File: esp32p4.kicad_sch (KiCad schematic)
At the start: 19 parts, among them U3 TLV62569DBV

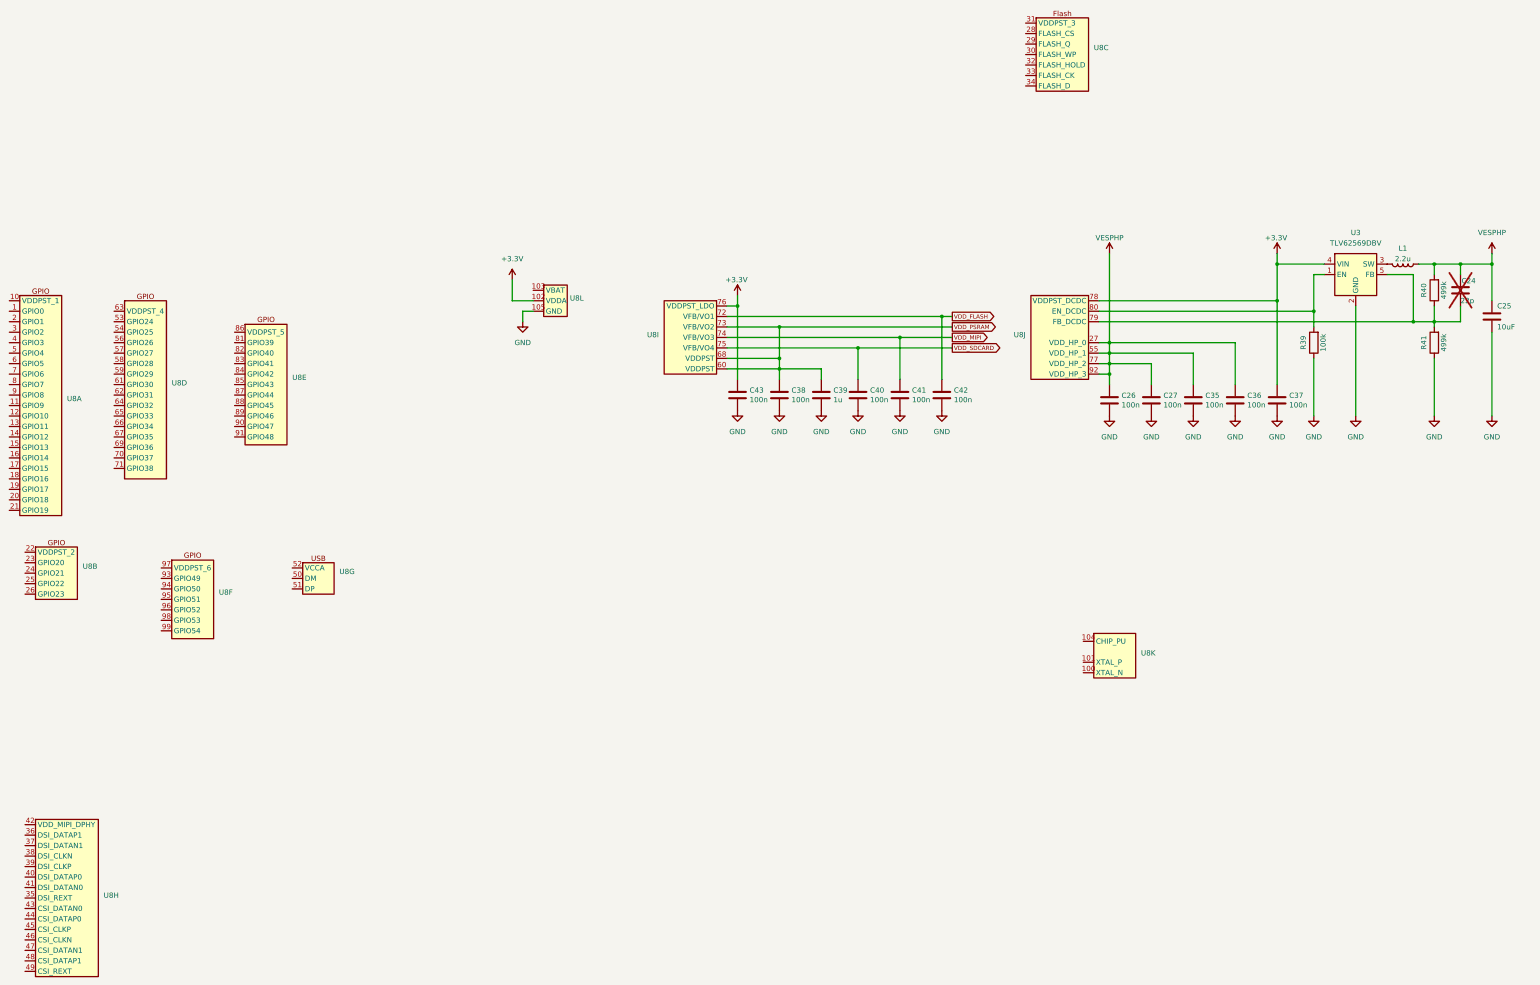
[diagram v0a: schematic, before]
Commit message: Mostly power related stuff for the ESP32-P4
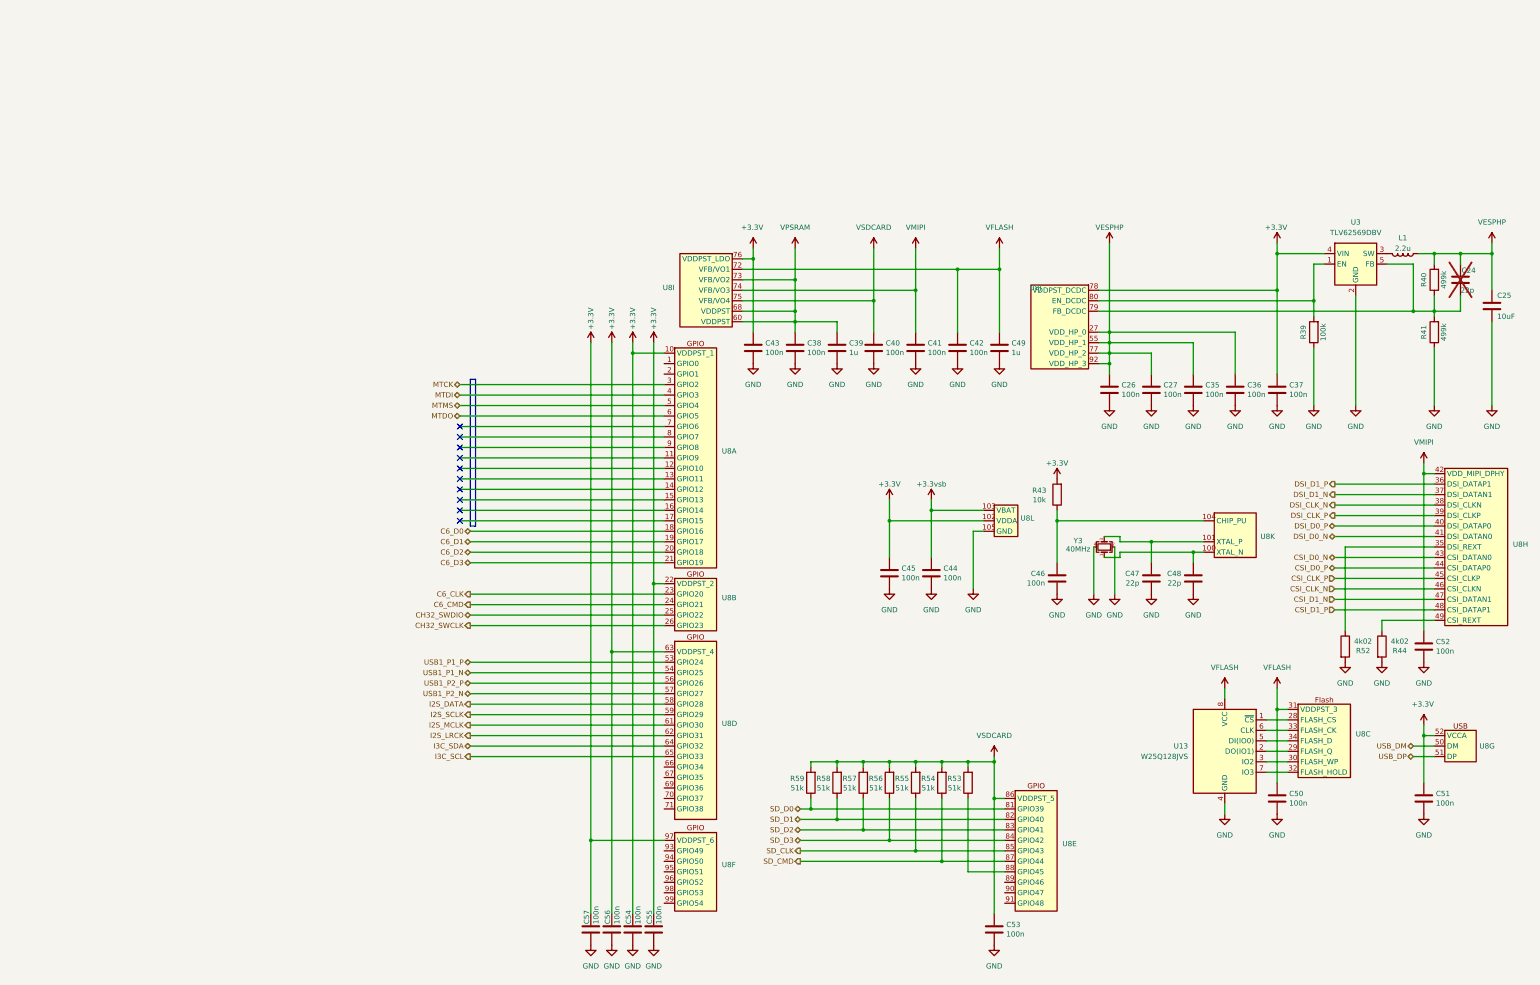
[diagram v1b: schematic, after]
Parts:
- added C44, C45, C46, C50, C51, C52, C53, C54, C55, C56, C57: 100n, Capacitor_SMD:C_0402_1005Metric, symbol symbols:C
- added C47, C48: 22p, Capacitor_SMD:C_0402_1005Metric, symbol symbols:C
- added C49: 1u, Capacitor_SMD:C_0402_1005Metric, symbol symbols:C
- added R43: 10k, Resistor_SMD:R_0402_1005Metric, symbol Device:R
- added R44, R52: 4k02, Resistor_SMD:R_0402_1005Metric, symbol Device:R
- added R53, R54, R55, R56, R57, R58, R59: 51k, Resistor_SMD:R_0402_1005Metric, symbol Device:R
- added U13: W25Q128JVS, Package_SO:SOIC-8_5.23x5.23mm_P1.27mm, symbol Memory_Flash:W25Q128JVS
- added Y3: 40MHz, symbol Device:Crystal_GND24_Small
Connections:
- net VDD_FLASH is gone; now on net VFLASH: C42.1, U8.72 (VFB/VO1)
- net VDD_MIPI is gone; now on net VMIPI: C41.1, U8.74 (VFB/VO3)
- net VDD_SDCARD is gone; now on net VSDCARD: C40.1, U8.75 (VFB/VO4)
- net +3.3V: now also U8.10 (VDDPST_1), U8.22 (VDDPST_2), U8.52 (VCCA), U8.63 (VDDPST_4), U8.97 (VDDPST_6), C45.1, C51.1, C54.1, C55.1, C56.1, C57.1, R43.2
- net GND: now also C44.2, C45.2, C46.2, C47.2, C48.2, C49.2, C50.2, C51.2, C52.2, C53.2, C54.2, C55.2, C56.2, C57.2, R44.2, R52.2, U13.4 (GND), Y3.2, Y3.4
- net at U8.35 (DSI_REXT): now also R52.1
- net DSI_D1_P: now reaches U8.36 (DSI_DATAP1)
- net DSI_D1_N: now reaches U8.37 (DSI_DATAN1)
- net DSI_CLK_N: now reaches U8.38 (DSI_CLKN)
- net DSI_CLK_P: now reaches U8.39 (DSI_CLKP)
- net DSI_D0_P: now reaches U8.40 (DSI_DATAP0)
- net DSI_D0_N: now reaches U8.41 (DSI_DATAN0)
- net VMIPI: now reaches U8.42 (VDD_MIPI_DPHY)
- net VMIPI: now also C52.1
- net CSI_D0_N: now reaches U8.43 (CSI_DATAN0)
- net CSI_D0_P: now reaches U8.44 (CSI_DATAP0)
- net CSI_CLK_P: now reaches U8.45 (CSI_CLKP)
- net CSI_CLK_N: now reaches U8.46 (CSI_CLKN)
- net CSI_D1_N: now reaches U8.47 (CSI_DATAN1)
- net CSI_D1_P: now reaches U8.48 (CSI_DATAP1)
- net at U8.49 (CSI_REXT): now also R44.1
- net C6_CLK: now reaches U8.23 (GPIO20)
- net C6_CMD: now reaches U8.24 (GPIO21)
- net CH32_SWDIO: now reaches U8.25 (GPIO22)
- net CH32_SWCLK: now reaches U8.26 (GPIO23)
- net at U8.28 (FLASH_CS): now also U13.1 (~{CS})
- net at U8.29 (FLASH_Q): now also U13.2 (DO(IO1))
- net at U8.30 (FLASH_WP): now also U13.3 (IO2)
- net VFLASH: now reaches U8.31 (VDDPST_3)
- net VFLASH: now also C49.1, C50.1, U13.8 (VCC)
- net at U8.32 (FLASH_HOLD): now also U13.7 (IO3)
- net at U8.33 (FLASH_CK): now also U13.6 (CLK)
- net at U8.34 (FLASH_D): now also U13.5 (DI(IO0))
- net C6_D0: now reaches U8.18 (GPIO16)
- net C6_D1: now reaches U8.19 (GPIO17)
- net C6_D2: now reaches U8.20 (GPIO18)
- net C6_D3: now reaches U8.21 (GPIO19)
- net MTCK: now reaches U8.3 (GPIO2)
- net MTDI: now reaches U8.4 (GPIO3)
- net MTMS: now reaches U8.5 (GPIO4)
- net MTDO: now reaches U8.6 (GPIO5)
- net USB_DM: now reaches U8.50 (DM)
- net USB_DP: now reaches U8.51 (DP)
- net +3.3vsb: now reaches U8.103 (VBAT)
- net +3.3vsb: now also C44.1
- net SD_D0: now reaches U8.81 (GPIO39)
- net SD_D0: now also R59.1
- net SD_D1: now reaches U8.82 (GPIO40)
- net SD_D1: now also R58.1
- net SD_D2: now reaches U8.83 (GPIO41)
- net SD_D2: now also R57.1
- net SD_D3: now reaches U8.84 (GPIO42)
- net SD_D3: now also R56.1
- net SD_CLK: now reaches U8.85 (GPIO43)
- net SD_CLK: now also R55.1
- net VSDCARD: now reaches U8.86 (VDDPST_5)
- net VSDCARD: now also C53.1, R53.2, R54.2, R55.2, R56.2, R57.2, R58.2, R59.2
- net SD_CMD: now reaches U8.87 (GPIO44)
- net SD_CMD: now also R54.1
- net at U8.88 (GPIO45): now also R53.1
- net USB1_P1_P: now reaches U8.53 (GPIO24)
- net USB1_P1_N: now reaches U8.54 (GPIO25)
- net USB1_P2_P: now reaches U8.56 (GPIO26)
- net USB1_P2_N: now reaches U8.57 (GPIO27)
- net I2S_DATA: now reaches U8.58 (GPIO28)
- net I2S_SCLK: now reaches U8.59 (GPIO29)
- net I2S_MCLK: now reaches U8.61 (GPIO30)
- net I2S_LRCK: now reaches U8.62 (GPIO31)
- net I3C_SDA: now reaches U8.64 (GPIO32)
- net I3C_SCL: now reaches U8.65 (GPIO33)
- net at U8.100 (XTAL_N): now also C48.1, Y3.1
- net at U8.101 (XTAL_P): now also C47.1, Y3.3
- net at U8.104 (CHIP_PU): now also C46.1, R43.1
- net VDD_PSRAM renamed VPSRAM
- no-connect marks 0 -> 10
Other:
- moved on the sheet: C24, C25, C26, C27, C35, C36, C37, C38, C39, C40, C41, C42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

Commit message: More schematics
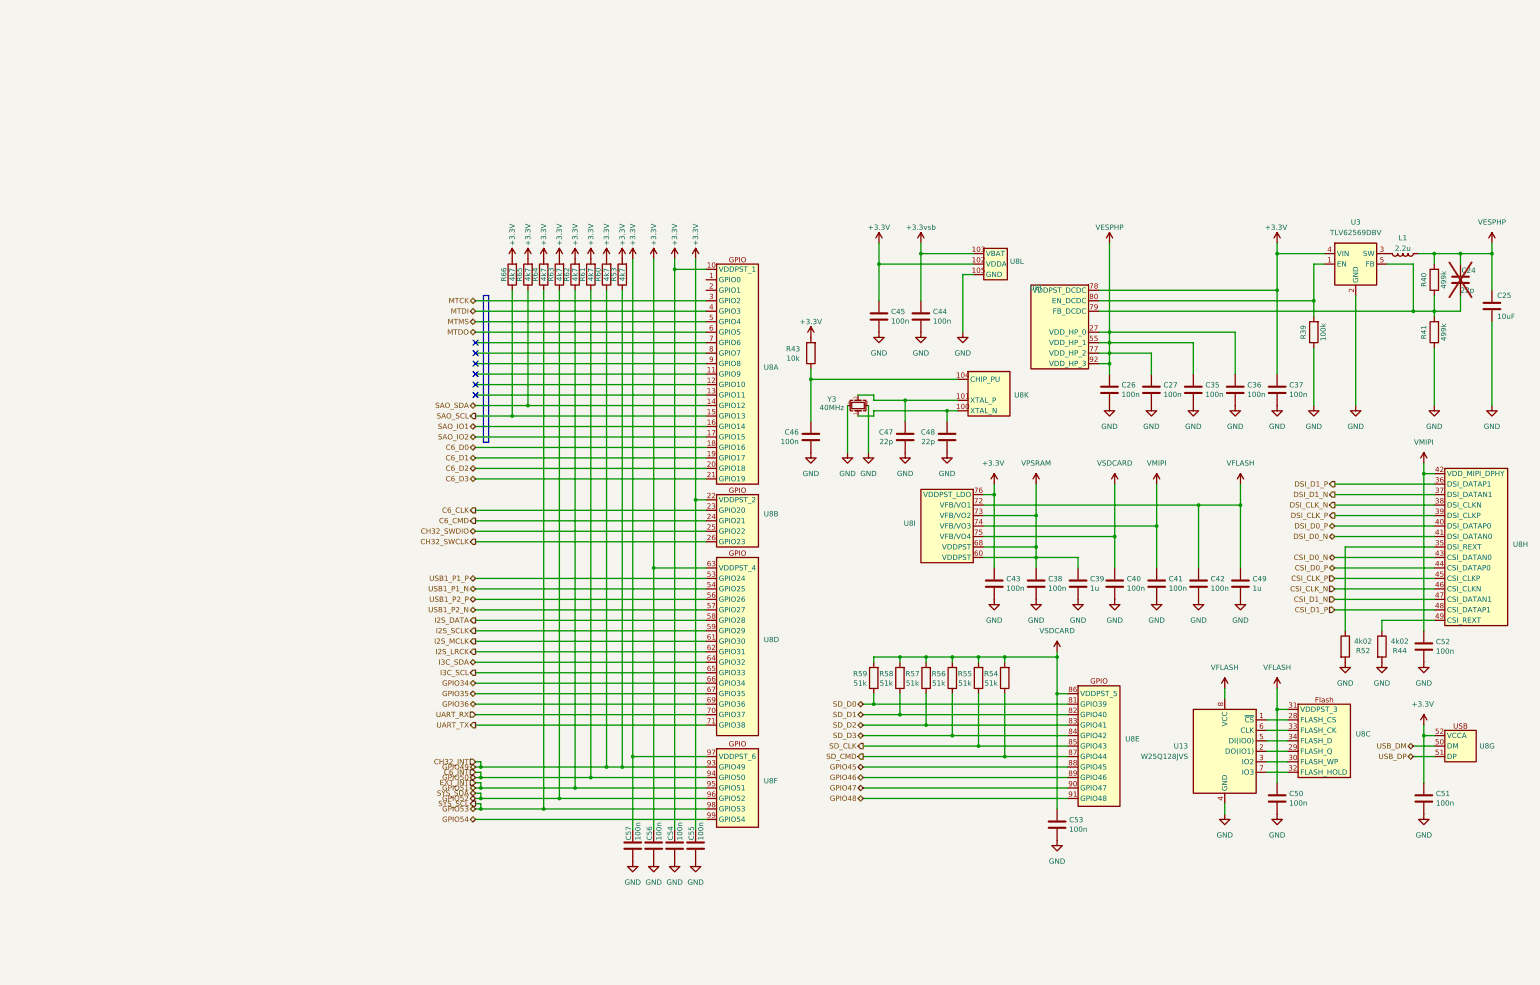
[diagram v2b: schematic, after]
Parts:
- added R60, R61, R62, R63, R64, R65, R66: 4k7, Resistor_SMD:R_0402_1005Metric, symbol Device:R
- R53: value 51k -> 4k7
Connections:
- net +3.3V: now also R53.2, R60.2, R61.2, R62.2, R63.2, R64.2, R65.2, R66.2
- net VSDCARD: no longer R53.2
- net CH32_INT: now reaches R53.1
- net CH32_INT: now also U8.93 (GPIO49), R60.1; no longer U8.88 (GPIO45)
- net C6_INT: now reaches U8.94 (GPIO50)
- net C6_INT: now also R61.1
- net EXT_INT: now reaches U8.95 (GPIO51)
- net EXT_INT: now also R62.1
- net GPIO52: now reaches U8.96 (GPIO52)
- net GPIO52: now also R63.1
- net GPIO53: now reaches U8.98 (GPIO53)
- net GPIO53: now also R64.1
- net GPIO54: now reaches U8.99 (GPIO54)
- net SAO_SDA: now reaches U8.14 (GPIO12)
- net SAO_SDA: now also R65.1
- net SAO_SCL: now reaches U8.15 (GPIO13)
- net SAO_SCL: now also R66.1
- net SAO_IO1: now reaches U8.16 (GPIO14)
- net SAO_IO2: now reaches U8.17 (GPIO15)
- net GPIO46: now reaches U8.89 (GPIO46)
- net GPIO47: now reaches U8.90 (GPIO47)
- net GPIO48: now reaches U8.91 (GPIO48)
- net GPIO34: now reaches U8.66 (GPIO34)
- net GPIO35: now reaches U8.67 (GPIO35)
- net GPIO36: now reaches U8.69 (GPIO36)
- net UART_RX: now reaches U8.70 (GPIO37)
- net UART_TX: now reaches U8.71 (GPIO38)
- new net GPIO45: U8.88 (GPIO45)
- no-connect marks 10 -> 6
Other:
- moved on the sheet: C38, C39, C40, C41, C42, C43, C44, C45, C46, C47, C48, C49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
